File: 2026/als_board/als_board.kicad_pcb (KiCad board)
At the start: 2 copper layers, 60 x 8 mm, 18 parts, among them J1 MAIN, J2 i2c, J3 PROG, U1 GM7333, U2 ME6209A50M3G, U3 CH32V003JxMx, U4 MAX485E

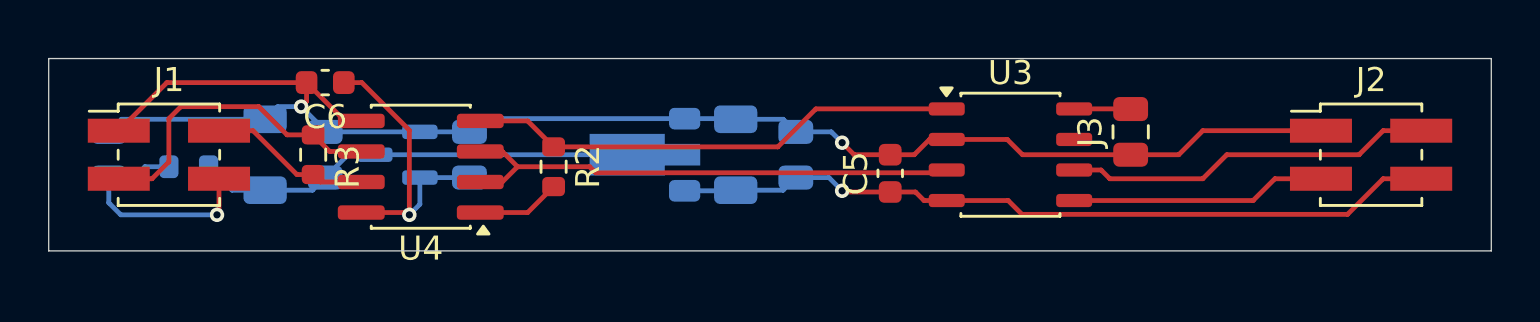
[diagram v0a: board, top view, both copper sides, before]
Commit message: ALS finishing touches
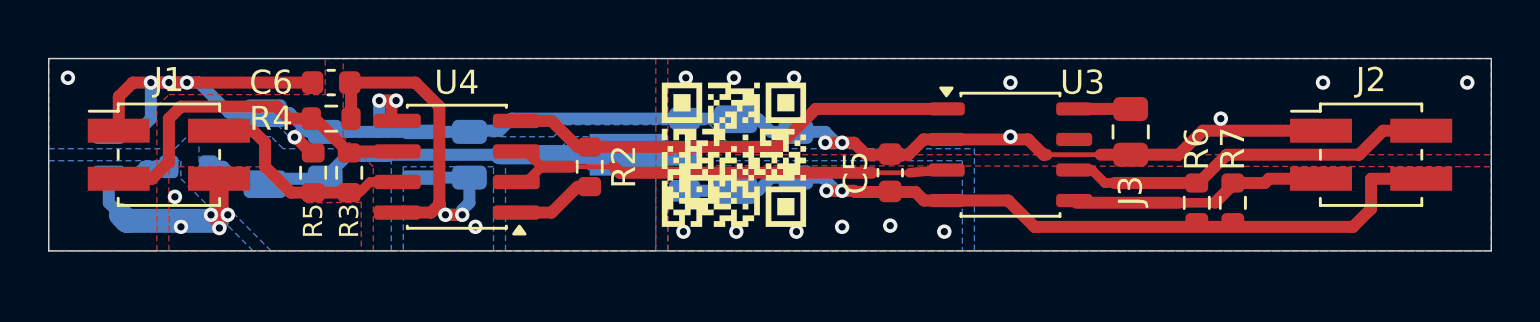
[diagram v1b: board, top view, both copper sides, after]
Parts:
- added G***: LOGO, MAGLab_Logo:MAGLab_Website_Small, F.Cu at (128.5, 105.0)
- added G***: LOGO, MAGLab_Logo:MAGLab_Symbol_Fine, B.Cu at (137.7, 103.6)
- added R4: 5k1, Resistor_SMD:R_0603_1608Metric, F.Cu at (111.8, 103.5)
- added R5: 5k1, Resistor_SMD:R_0603_1608Metric, F.Cu at (111.0, 105.8)
- added R6: 10k, Resistor_SMD:R_0603_1608Metric, F.Cu at (147.8, 107.0)
- added R7: 10k, Resistor_SMD:R_0603_1608Metric, F.Cu at (149.2, 107.0)
- moved R3 1.68 mm to (112.5, 105.8)
- moved R2 1.50 mm to (122.5, 105.5)
- moved U4 1.50 mm to (117.0, 105.5)
- moved C1 0.25 mm to (109.0, 104.8)
- moved C6 0.25 mm to (111.8, 102.0)
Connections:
- net Net-(J2-Pin_2) renamed /SCL
- net Net-(J2-Pin_3) renamed /SDA
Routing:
- net +5V: track 12.9 -> 18.5 mm, vias 1 -> 3
- net GND: track 65.8 -> 69.7 mm, vias 2 -> 17
- net /12V_FIL: track 20.7 -> 23.4 mm
- net Net-(J1-Pin_2): track 6.80 -> 9.10 mm
- net +3V3: track 32.1 -> 34.2 mm, vias 1 -> 8
- net Net-(J1-Pin_3): track 13.2 -> 14.7 mm
- net Net-(U3-PD6/PA1): track 20.5 -> 19.5 mm
- net Net-(U3-PA2): track 21.6 -> 20.7 mm
- net +12V: track 10.0 -> 10.7 mm, vias 1 -> 5
- added copper zone on B.Cu, net +12V
- added copper zone on F.Cu, net +12V
- added copper zone on B.Cu, net +3V3
- added copper zone on F.Cu, net +3V3
- added copper zone on B.Cu, net +5V
- added copper zone on F.Cu, net +5V
- added copper zone on B.Cu, net /12V_FIL
- added copper zone on B.Cu, net GND
- added copper zone on F.Cu, net GND
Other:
- board text added: "${TITLE}"
- board text added: "Rev. ${REVISION}"
